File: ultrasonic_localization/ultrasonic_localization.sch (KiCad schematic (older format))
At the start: 6 parts

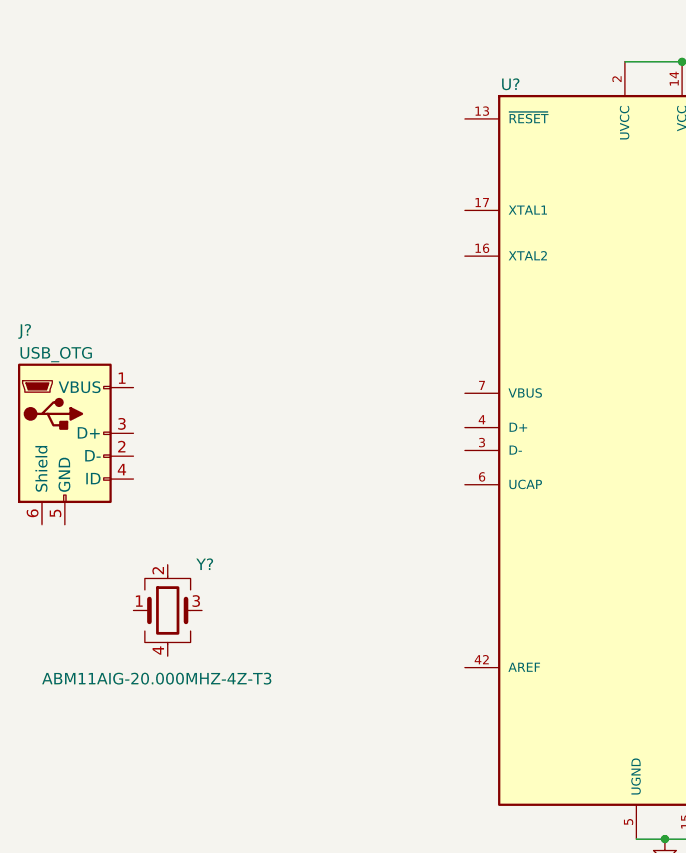
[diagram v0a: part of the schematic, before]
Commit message: updated oscillator connections
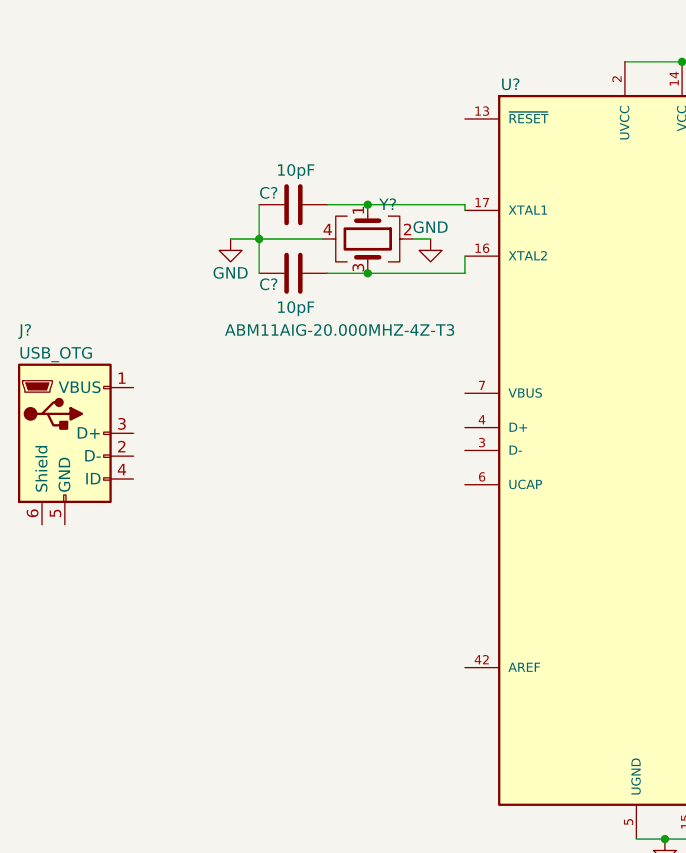
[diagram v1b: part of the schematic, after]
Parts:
- added C? (x2): 10pF, symbol C
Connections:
- net GND: now also Y?.2, Y?.4, C?.2, C?.2
- net at U?.16 (XTAL2): now also Y?.3, C?.1
- net at U?.17 (XTAL1): now also Y?.1, C?.1
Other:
- moved on the sheet: Y?
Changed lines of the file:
@@
 L Crystal_GND24 Y?
 U 1 1 59F78768
-P 2275 3950
-F 0 "Y?" H 2400 4150 50  0000 L CNN
-F 1 "ABM11AIG-20.000MHZ-4Z-T3" H 1725 3650 50  0000 L CNN
-F 2 "Crystals:Crystal_SMD_2016-4pin_2.0x1.6mm" H 2275 3950 50  0001 C CNN
-F 3 "" H 2275 3950 50  0001 C CNN
-	1    2275 3950
-	1    0    0    -1
+P 3150 2325
+F 0 "Y?" V 3000 2375 50  0000 L CNN
+F 1 "ABM11AIG-20.000MHZ-4Z-T3" V 3550 1700 50  0000 L CNN
+F 2 "Crystals:Crystal_SMD_2016-4pin_2.0x1.6mm" H 3150 2325 50  0001 C CNN
+F 3 "" H 3150 2325 50  0001 C CNN
+	1    3150 2325
+	0    1    1    0
 $EndComp
 $Comp
@@
 	1    0    0    -1
 $EndComp
+$Comp
+L GND #PWR?
+U 1 1 59F78D8A
+P 3425 2325
+F 0 "#PWR?" H 3425 2075 50  0001 C CNN
+F 1 "GND" H 3425 2375 50  0000 C CNN
+F 2 "" H 3425 2325 50  0001 C CNN
+F 3 "" H 3425 2325 50  0001 C CNN
+	1    3425 2325
+	1    0    0    -1
+$EndComp
+Wire Wire Line
+	3350 2325 3425 2325
+$Comp
+L GND #PWR?
+U 1 1 59F78F19
+P 2550 2325
+F 0 "#PWR?" H 2550 2075 50  0001 C CNN
+F 1 "GND" H 2550 2175 50  0000 C CNN
+F 2 "" H 2550 2325 50  0001 C CNN
+F 3 "" H 2550 2325 50  0001 C CNN
+	1    2550 2325
+	1    0    0    -1
+$EndComp
+$Comp
+L C C?
+U 1 1 59F78F38
+P 2825 2475
+F 0 "C?" V 2875 2325 50  0000 L CNN
+F 1 "10pF" V 2975 2400 50  0000 L CNN
+F 2 "" H 2863 2325 50  0001 C CNN
+F 3 "" H 2825 2475 50  0001 C CNN
+	1    2825 2475
+	0    1    1    0
+$EndComp
+$Comp
+L C C?
+U 1 1 59F7904A
+P 2825 2175
+F 0 "C?" V 2775 2025 50  0000 L CNN
+F 1 "10pF" V 2675 2100 50  0000 L CNN
+F 2 "" H 2863 2025 50  0001 C CNN
+F 3 "" H 2825 2175 50  0001 C CNN
+	1    2825 2175
+	0    1    1    0
+$EndComp
+Wire Wire Line
+	2975 2475 3575 2475
+Wire Wire Line
+	3575 2475 3575 2400
+Wire Wire Line
+	2975 2175 3575 2175
+Wire Wire Line
+	3575 2175 3575 2200
+Connection ~ 3150 2175
+Connection ~ 3150 2475
+Wire Wire Line
+	2950 2325 2550 2325
+Wire Wire Line
+	2675 2175 2675 2475
+Connection ~ 2675 2325
 $EndSCHEMATC
